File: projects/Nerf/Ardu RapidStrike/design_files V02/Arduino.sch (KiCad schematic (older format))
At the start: 73 parts, among them J1 BATT_OUT, J10 PWM_IN, J11 PWM_OUT, J12 CLIP, J14 NPTH, J15 BATT, J16 NPTH, J17 PSH_IN, J18 PSH_OUT, J19 TRIG, J2 BATT_IN, J20 PUSH, J21 BUTTON, J22 TRIG_OUT, J23 TRIG_IN, J24 TO_IR, J25 PHOTO, J26 IR_LED, J27 BUTTON, J3 PUSHER, J4 JAM, J5 I2C, J6 REV, J7 FTDI, J8 PHOTO, J9 FLYWHEELS, Q1 IRLB8721, Q2 Photo_NPN, SW1 SW_Rotary8, SW2 SW_Push, U1 MCP1702, U2 L293D, U3 HALL SENSOR, U4 HALL SENSOR, U5 ATMEGA328P-PU, U6 HALL SENSOR, U7 74LS14, Y1 16Mhz

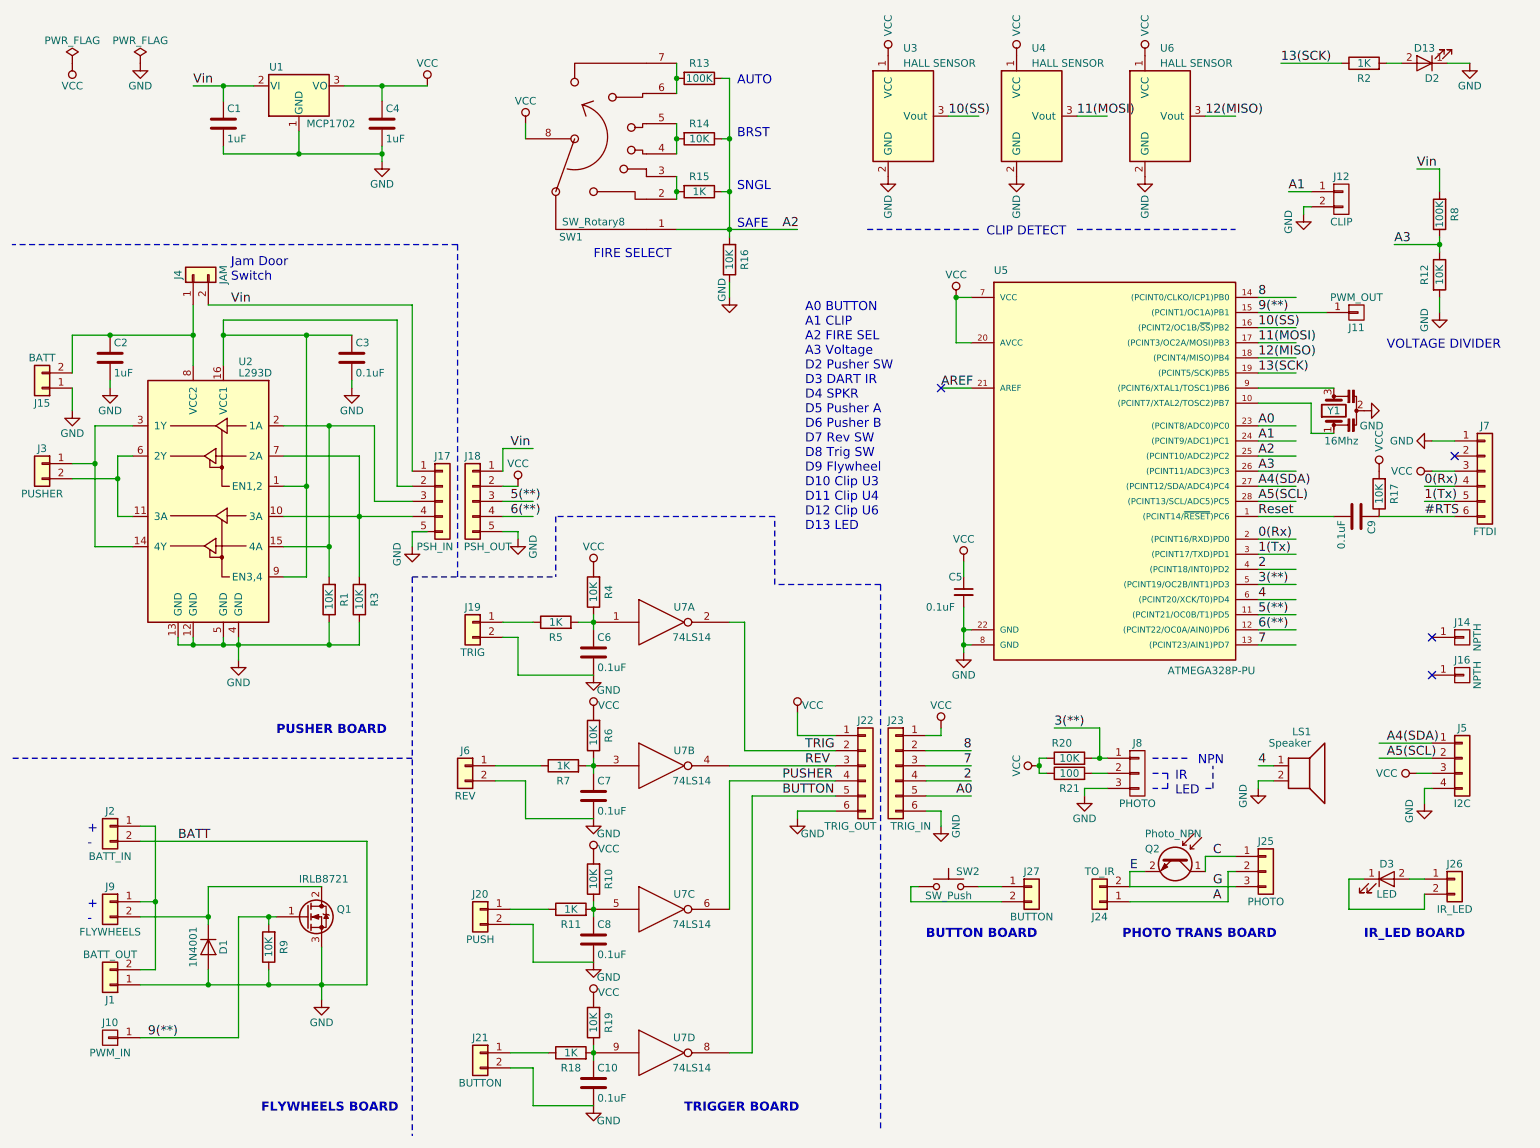
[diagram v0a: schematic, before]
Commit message: Updates
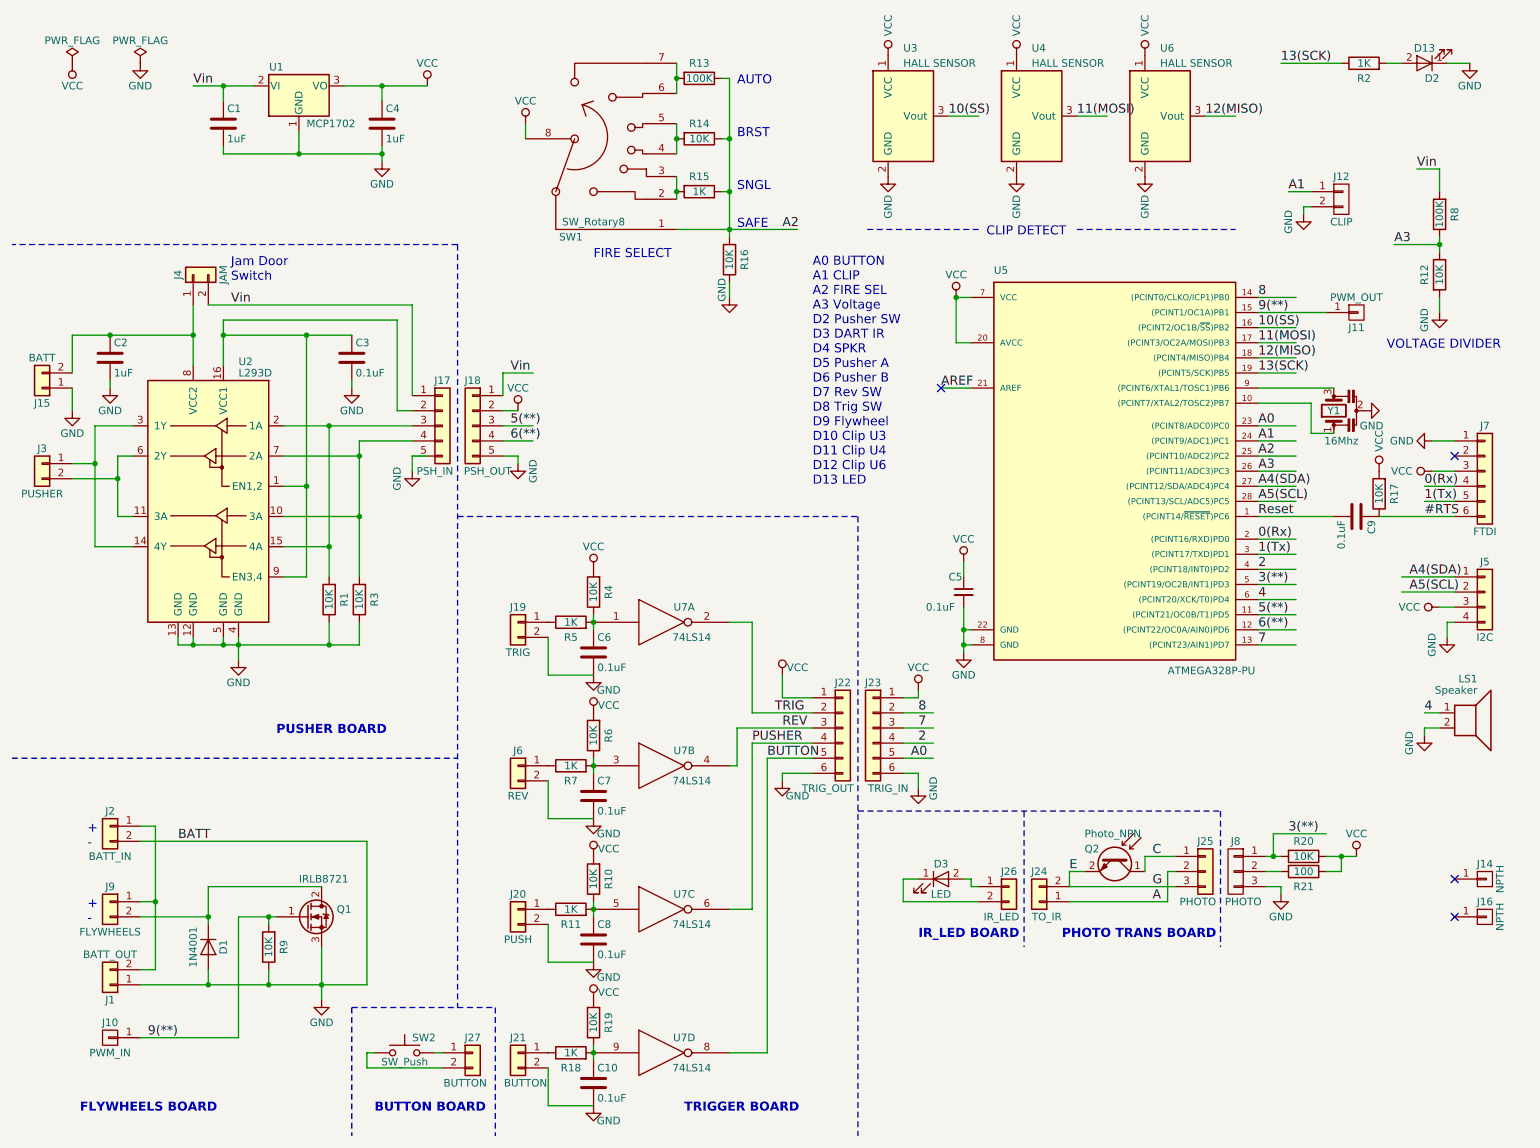
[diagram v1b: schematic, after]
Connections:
- wire segments 215 -> 211
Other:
- note removed: "IR\nLED"
- note removed: "NPN"
- moved on the sheet: D3, J14, J16, J17, J18, J19, J20, J21, J22, J23, J24, J25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
